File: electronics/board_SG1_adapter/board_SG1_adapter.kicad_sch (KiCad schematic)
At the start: 25 parts, among them J1 Conn_01x01, J2 Conn_01x01, J3 Conn_01x03, J4 Conn_01x03, T1 10P_1P_2S

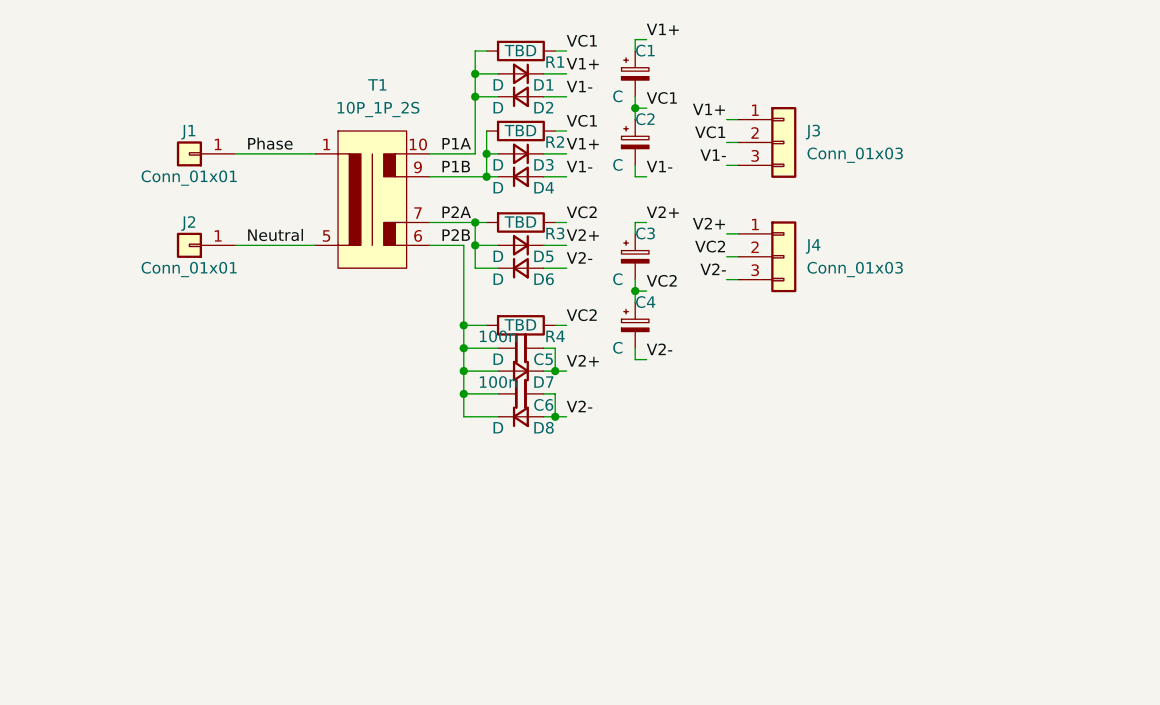
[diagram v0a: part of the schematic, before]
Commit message: WIP further development
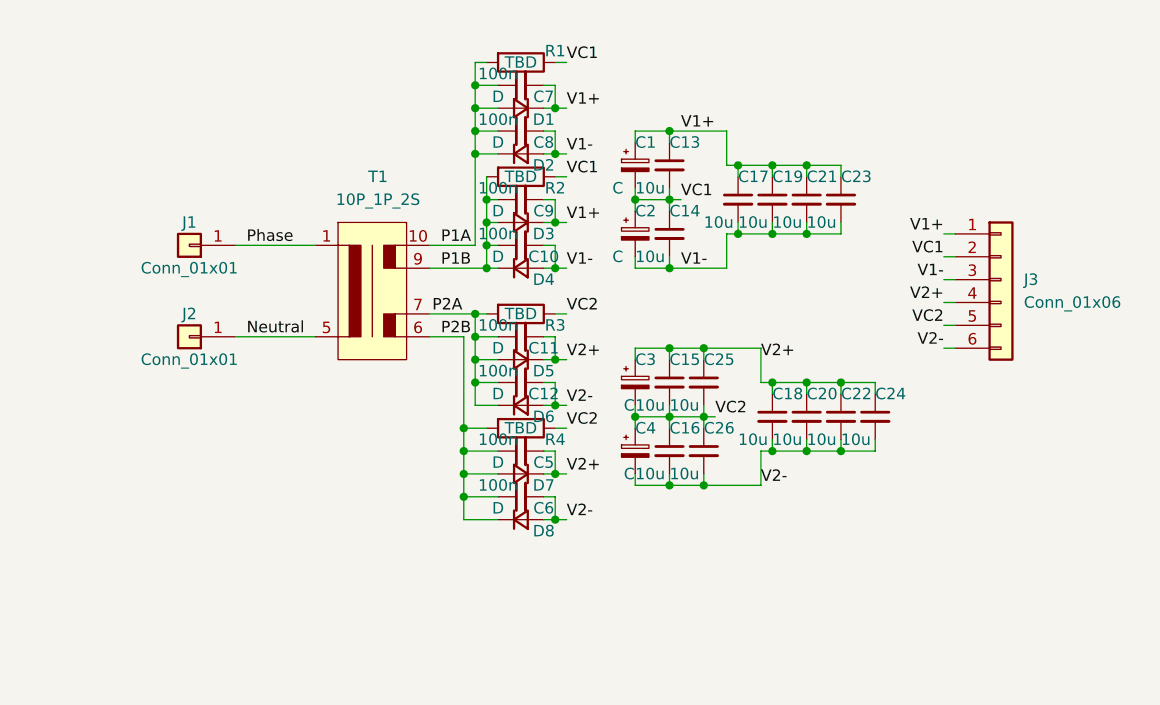
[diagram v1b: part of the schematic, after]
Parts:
- removed J3, J4: Conn_01x03, symbol Connector_Generic:Conn_01x03
- added C10, C11, C12, C7, C8, C9: 100n, SquantorRcl:C_0805+0603, symbol Device:C_Small
- added C13, C14, C15, C16, C17, C18, C19, C20, C21, C22, C23, C24, C25, C26: 10u, SquantorRcl:C_1206_0805, symbol Device:C_Small
- added J3: Conn_01x06, Connector_Molex:Molex_KK-254_AE-6410-06A_1x06_P2.54mm_Vertical, symbol Connector_Generic:Conn_01x06
- C1, C2, C3, C4: footprint SquantorRcl:C-050-075-100-elco -> SquantorRcl:C-050-100-elco
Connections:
- net P1A: now also C7.1, C8.1
- net P1B: now also C10.1, C9.1
- net P2A: now also C11.1, C12.1
- net V1+: now also C13.1, C17.1, C19.1, C21.1, C23.1, C7.2, C9.2, J3.1 (Pin_1)
- net V1-: now also C10.2, C14.2, C17.2, C19.2, C21.2, C23.2, C8.2, J3.3 (Pin_3)
- net V2+: now also C11.2, C15.1, C18.1, C20.1, C22.1, C24.1, C25.1, J3.4 (Pin_4)
- net V2-: now also C12.2, C16.2, C18.2, C20.2, C22.2, C24.2, C26.2, J3.6 (Pin_6)
- net VC1: now also C13.2, C14.1, J3.2 (Pin_2)
- net VC2: now also C15.2, C16.1, C25.2, C26.1, J3.5 (Pin_5)
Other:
- moved on the sheet: C1, C2, C3, C4, C5, C6, D1, D2, D3, D4, D5, D6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
